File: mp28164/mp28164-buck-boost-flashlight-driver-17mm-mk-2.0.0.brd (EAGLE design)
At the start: 25 x 16 mm, 30 parts, among them J1 AVR_SPI_PRG_6PTH, U1 MPS28164, U2 ATTINY25-20MU, U3 OPA399, U4 V_REG_ENTLV700

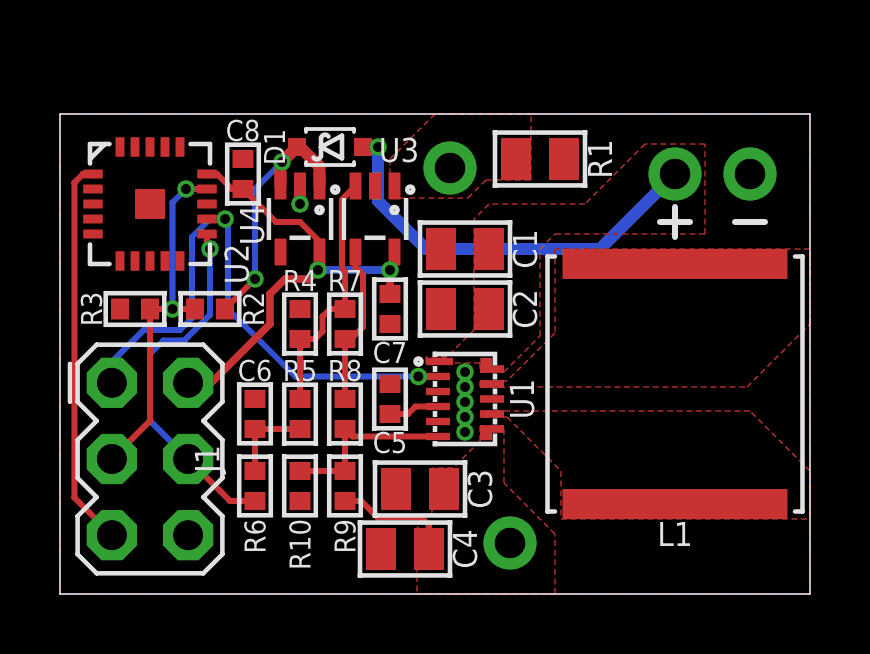
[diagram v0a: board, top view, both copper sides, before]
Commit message: whole bunch of crap in here
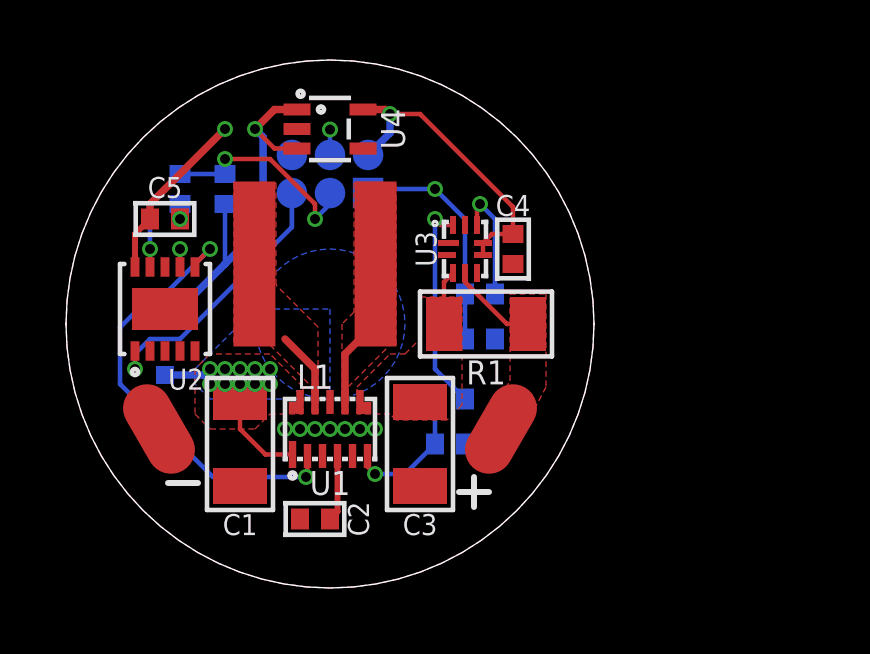
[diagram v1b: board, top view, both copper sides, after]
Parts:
- removed C8: 1uF, a_parts:C0402
- removed IN+, IN-: M01PTH-1MM-CIR-NS, a_parts:1X01-1MM-CIR-NS
- removed R10: 68k, a_parts:R0402
- removed R5: 360k, a_parts:R0402
- removed R7: 75k, a_parts:R0402
- removed R8: 1k, a_parts:R0402
- removed R9: 750k, a_parts:R0402
- +, -: value M01PTH-1MM-CIR-NS -> M01SMD-1.6MMX3.2MM-NS; device a_parts:1X01-1MM-CIR-NS -> a_parts:1X01-SMD-1.6MMX3.2MM-NS
- C1: value 10uF -> 22uF; device a_parts:C0805-TIGHTER -> a_parts:C1206
- C2: value 10uF -> 100nF; device a_parts:C0805-TIGHTER -> a_parts:C0402
- C3: value 22uF -> 47uF; device a_parts:C0805-TIGHTER -> a_parts:C1206
- C4: value 22uF -> 1uF; device a_parts:C0805-TIGHTER -> a_parts:C0402
- C5: value 100nF -> 1uF
- C6: value 6800pF -> 1nF
- C7: value 1uF -> 1nF
- J1: value AVR_SPI_PRG_6PTH -> AVR_SPI_PRG_6SMD-1.27MM; device a_parts:2X3 -> a_parts:2X3-1.27MM-SMD
- L1: value 2.2uH -> 1uH; device a_parts:XAR7030 -> a_parts:XAL60XX
- R1: device a_parts:R0805-TIGHTER -> a_parts:R1206
- R4: value 4.7k -> 6.8k
- R6: value 1k -> 6.8k
- U2: value ATTINY25-20MU -> ATTINY1310M1; device a_parts:QFN20 -> a_parts:QFN10(2X5)
- U3: value OPA399 -> INA190RSW; device a_parts:SC70 -> a_parts:UQFN-10
- moved - 13.0 mm to (3.30, 5.50), turned to 210 degrees
- moved L1 12.6 mm to (8.50, 11.0), turned to 0 degrees
- moved J1 11.2 mm to (9.00, 14.0), flipped to the bottom, turned to 0 degrees
- moved C4 10.6 mm to (15.1, 11.5), turned to 270 degrees
- moved C1 9.92 mm to (6.00, 5.00), turned to 270 degrees
- moved C5 9.60 mm to (3.50, 12.5), turned to 180 degrees
- moved C2 8.60 mm to (8.50, 2.50)
- moved D1 8.51 mm to (3.50, 8.40), flipped to the bottom, turned to 90 degrees
- moved R6 7.12 mm to (13.0, 6.50), flipped to the bottom, turned to 180 degrees
- moved C6 6.58 mm to (13.0, 5.00), flipped to the bottom, turned to 180 degrees
- moved R4 6.08 mm to (14.0, 10.0), flipped to the bottom, turned to 0 degrees
- moved R1 5.79 mm to (14.2, 9.00), turned to 0 degrees
- moved U1 4.61 mm to (9.00, 5.50), turned to 90 degrees
- moved R3 4.27 mm to (4.00, 13.5), flipped to the bottom, turned to 90 degrees
- moved R2 4.03 mm to (5.50, 13.5), flipped to the bottom, turned to 90 degrees
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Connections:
- removed net LED-: -.1, R1.2, U3.1
- removed net N$1: C6.1, R5.2, R6.2
- removed net OPAMP-: R4.2, R5.1, R7.1, U3.3
- removed net OPAMP_OUT: R7.2, R8.1, U3.4
- new net CSOUT: R6.2, U3.10
- new net LED+: +.P$1, R1.2, U3.4
- new net REF: R4.1, U3.8
- net ALTPWM/MOSI: now also U1.2, U2.6; no longer R6.1, U2.11
- net FB: now also C6.1, R6.1; no longer R10.2, R8.2, R9.2
- net GND: now also -.P$1, U2.5, U3.9; no longer C8.1, IN-.1, R1.1, R10.1, R4.1, U2.8, U3.2
- net PWM/MISO: now also C7.2, R4.2, U2.7; no longer U1.2, U2.12
- net VBAT: no longer C2.1, IN+.1
- net VCC: now also C4.1, C5.2, U2.10, U3.6, U3.7; no longer C7.2, C8.2, U2.15, U3.5
- net VDD: now also C2.1; no longer C5.2
- net VDIV/SCK: now also U2.9; no longer U2.14
- net VOUT: now also R1.1, U3.3; no longer +.1, C4.1, R9.1
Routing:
- net ALTPWM/MOSI: track 12.1 -> 21.5 mm, vias 1 -> 3
- net VBAT: track 13.9 -> 4.58 mm, vias 1 -> 10
- net OPAMP-: track 8.53 -> 0.00 mm
- net CSOUT: track 0.00 -> 7.10 mm, vias 0 -> 1
- net VCC: track 16.0 -> 22.4 mm
- net OPAMP_OUT: track 5.37 -> 0.00 mm
- net VBAT_RECT: track 8.88 -> 13.1 mm, vias 2 -> 1
- net REF: track 0.00 -> 3.95 mm, vias 0 -> 1
- net RST: track 13.0 -> 9.22 mm, vias 0 -> 1
- net LED+: track 0.00 -> 2.98 mm
- net N$1: track 2.90 -> 0.00 mm
- net L1: track 0.00 -> 2.51 mm
- net L2: track 0.00 -> 2.31 mm
- net VOUT: track 3.93 -> 1.82 mm
- net FB: track 6.10 -> 4.62 mm, vias 0 -> 1
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- added copper zone on layer 15, net GND
- added copper zone on layer 1, net LED+
- added copper zone on layer 16, net VBAT
- removed copper zone on layer 1, net LED-
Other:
- board size 25 x 16 mm -> 17.6 x 17.6 mm
- board text added: "LED Driver"
- board text added: "MP28614"
- board text removed: "MP28164 Buck-Boost LED Driver"
